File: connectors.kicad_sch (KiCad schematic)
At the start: 13 parts, among them J3 Serial Wire Debug, J4 JST-PH, J7 USB_C_Receptacle_USB2.0, J8 External UART, J9 External I2C, U2 USBLC6-2SC6

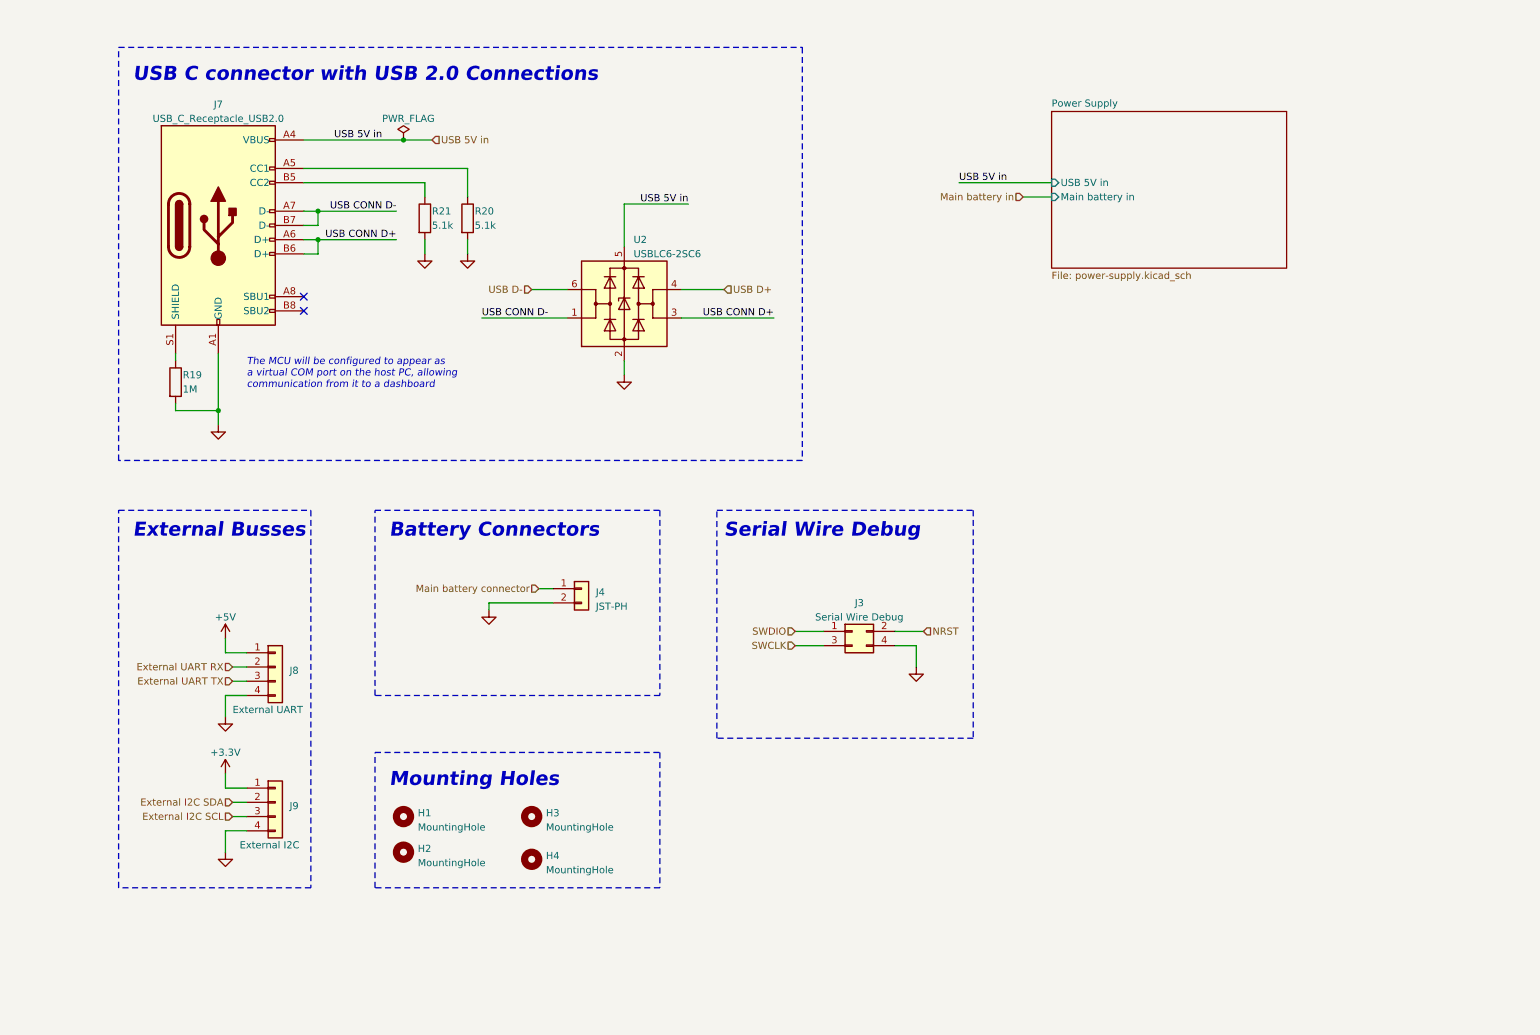
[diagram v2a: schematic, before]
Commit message: Updated with notes from Erik Welsh
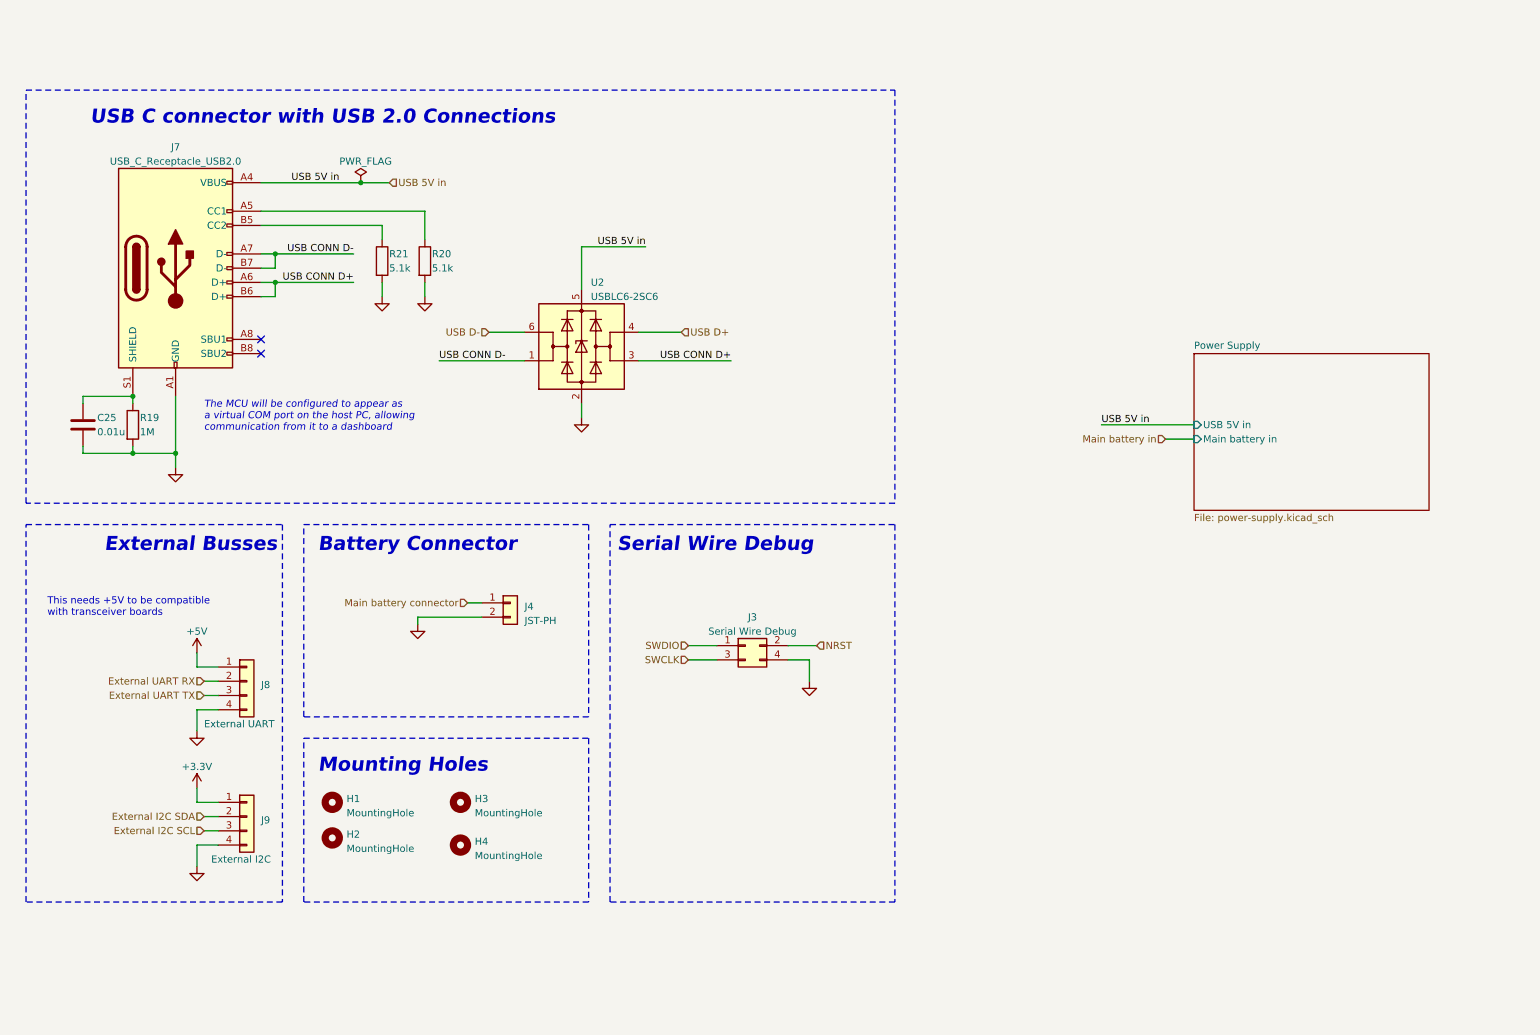
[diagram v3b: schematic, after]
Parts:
- added C25: 0.01u, Capacitor_SMD:C_0402_1005Metric, symbol Device:C
- H1, H2, H3, H4: footprint MountingHole:MountingHole_2mm -> MountingHole:MountingHole_2.2mm_M2
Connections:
- net GND: now also C25.2
- net at J7.S1 (SHIELD), R19.1: now also C25.1
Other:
- note added: "Battery Connector"
- note added: "This needs +5V to be compatible with transceiver boards"
- note removed: "Battery Connectors"
- moved on the sheet: H1, H2, H3, H4, J3, J4, J7, J8, J9, R19, R20, R21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
